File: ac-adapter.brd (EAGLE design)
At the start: 98.4 x 47 mm, 67 parts, among them IC1 BM1Q011, IC2 TL431, Q1 TLP621-1, Q2 600V5A, T1 COMMON_FILTER-SU10VFC, T2 TRANSFORMAER_FLYBACK-PQ2620-2

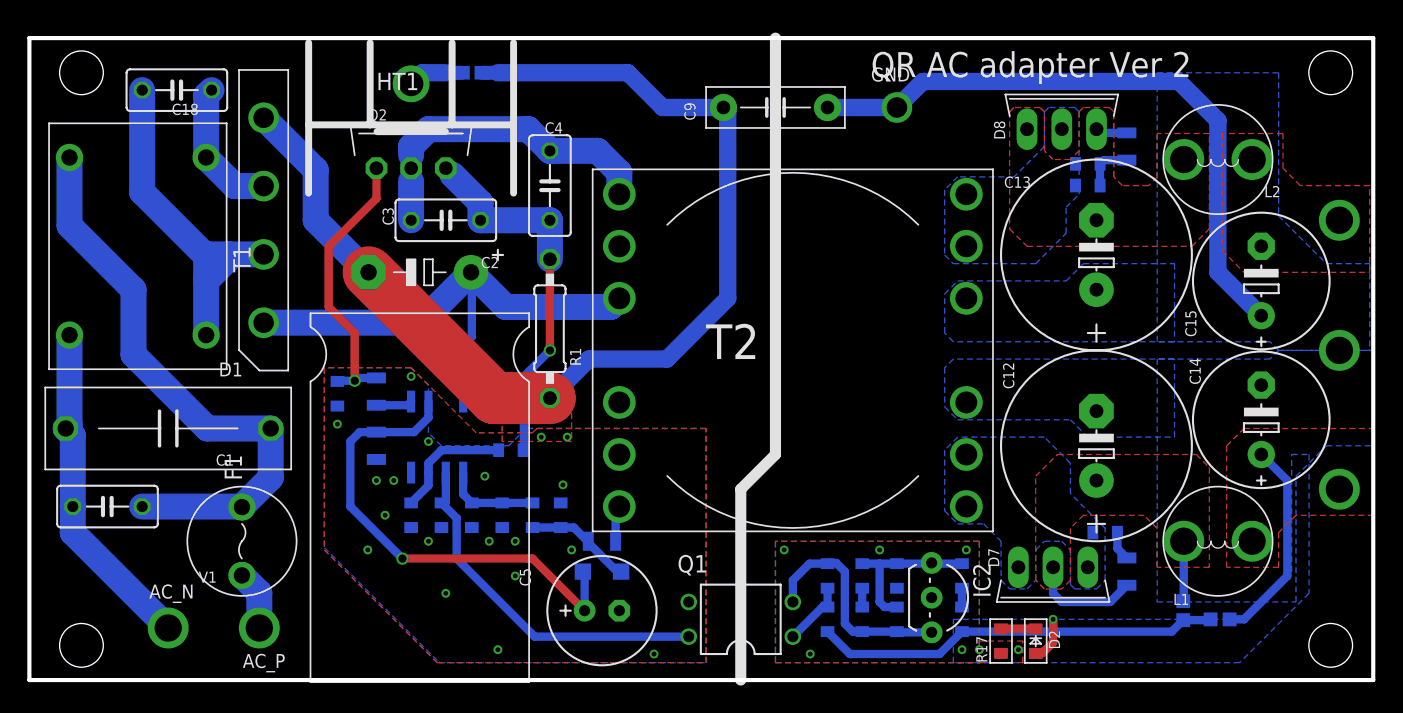
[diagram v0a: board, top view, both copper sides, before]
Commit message: 発注
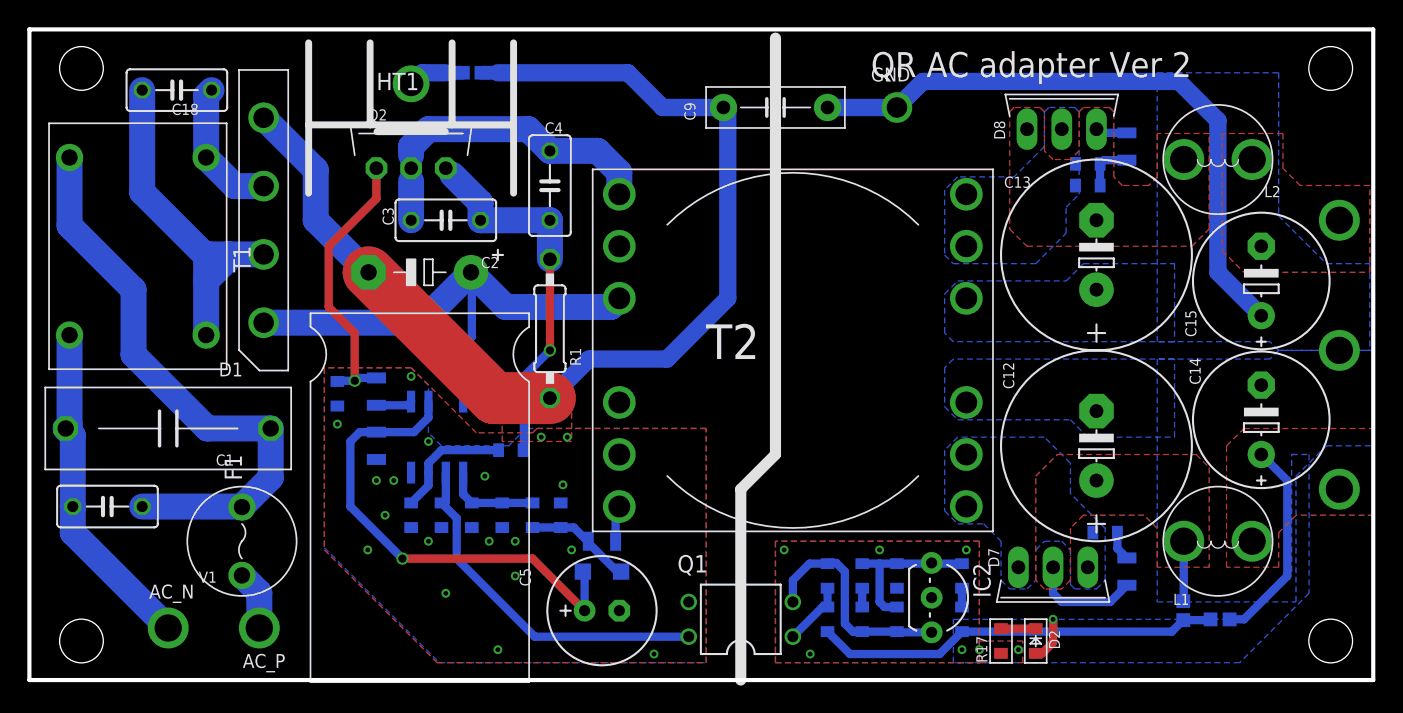
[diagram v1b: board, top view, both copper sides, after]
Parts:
- moved DR1 0.32 mm to (3.81, 2.86)
- moved DR3 0.32 mm to (95.2, 2.86)
- moved DR2 0.32 mm to (3.81, 44.8)
- moved DR4 0.32 mm to (95.2, 44.8)
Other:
- board size 98.4 x 47 mm -> 98.4 x 47.6 mm
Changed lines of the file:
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@@
 <board>
 <plain>
-<wire x1="0" y1="0" x2="0" y2="46.99" width="0.3048" layer="20"/>
-<wire x1="0" y1="46.99" x2="98.365" y2="46.99" width="0.3048" layer="20"/>
-<wire x1="98.365" y1="46.99" x2="98.365" y2="0" width="0.3048" layer="20"/>
+<wire x1="0" y1="0" x2="0" y2="47.625" width="0.3048" layer="20"/>
+<wire x1="0" y1="47.625" x2="98.365" y2="47.625" width="0.3048" layer="20"/>
+<wire x1="98.365" y1="47.625" x2="98.365" y2="0" width="0.3048" layer="20"/>
 <wire x1="98.365" y1="0" x2="0" y2="0" width="0.3048" layer="20"/>
 <text x="61.595" y="44.1325" size="1.8288" layer="21">QR AC adapter Ver 2</text>
-<dimension x1="0" y1="0" x2="0" y2="46.99" x3="-2.540003125" y3="23.495" textsize="1.778" layer="47"/>
+<dimension x1="0" y1="0" x2="0" y2="47.625" x3="-2.540003125" y3="23.8125" textsize="1.778" layer="47"/>
 <wire x1="52.07" y1="0" x2="52.07" y2="13.97" width="0.8128" layer="21"/>
 <wire x1="52.07" y1="13.97" x2="54.61" y2="16.51" width="0.8128" layer="21"/>
@@
 <attribute name="VALUE" x="20.47875" y="29.62275" size="1.016" layer="27" ratio="10" rot="R90"/>
 </element>
-<element name="DR1" library="my_connector" package="HOLE_3.2" value="HOLE-3.2" x="3.81" y="2.54" smashed="yes"/>
-<element name="DR2" library="my_connector" package="HOLE_3.2" value="HOLE-3.2" x="3.81" y="44.45" smashed="yes"/>
-<element name="DR3" library="my_connector" package="HOLE_3.2" value="HOLE-3.2" x="95.25" y="2.54" smashed="yes"/>
-<element name="DR4" library="my_connector" package="HOLE_3.2" value="HOLE-3.2" x="95.25" y="44.45" smashed="yes"/>
+<element name="DR1" library="my_connector" package="HOLE_3.2" value="HOLE-3.2" x="3.81" y="2.8575" smashed="yes"/>
+<element name="DR2" library="my_connector" package="HOLE_3.2" value="HOLE-3.2" x="3.81" y="44.7675" smashed="yes"/>
+<element name="DR3" library="my_connector" package="HOLE_3.2" value="HOLE-3.2" x="95.25" y="2.8575" smashed="yes"/>
+<element name="DR4" library="my_connector" package="HOLE_3.2" value="HOLE-3.2" x="95.25" y="44.7675" smashed="yes"/>
 <element name="C17" library="my_rcl" package="1608" value="1000p" x="38.89375" y="12.065" smashed="yes" rot="MR90">
 <attribute name="NAME" x="39.89375" y="10.465" size="0.8128" layer="26" rot="MR90"/>
